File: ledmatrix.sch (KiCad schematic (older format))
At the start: 62 parts, among them U58 sled1735

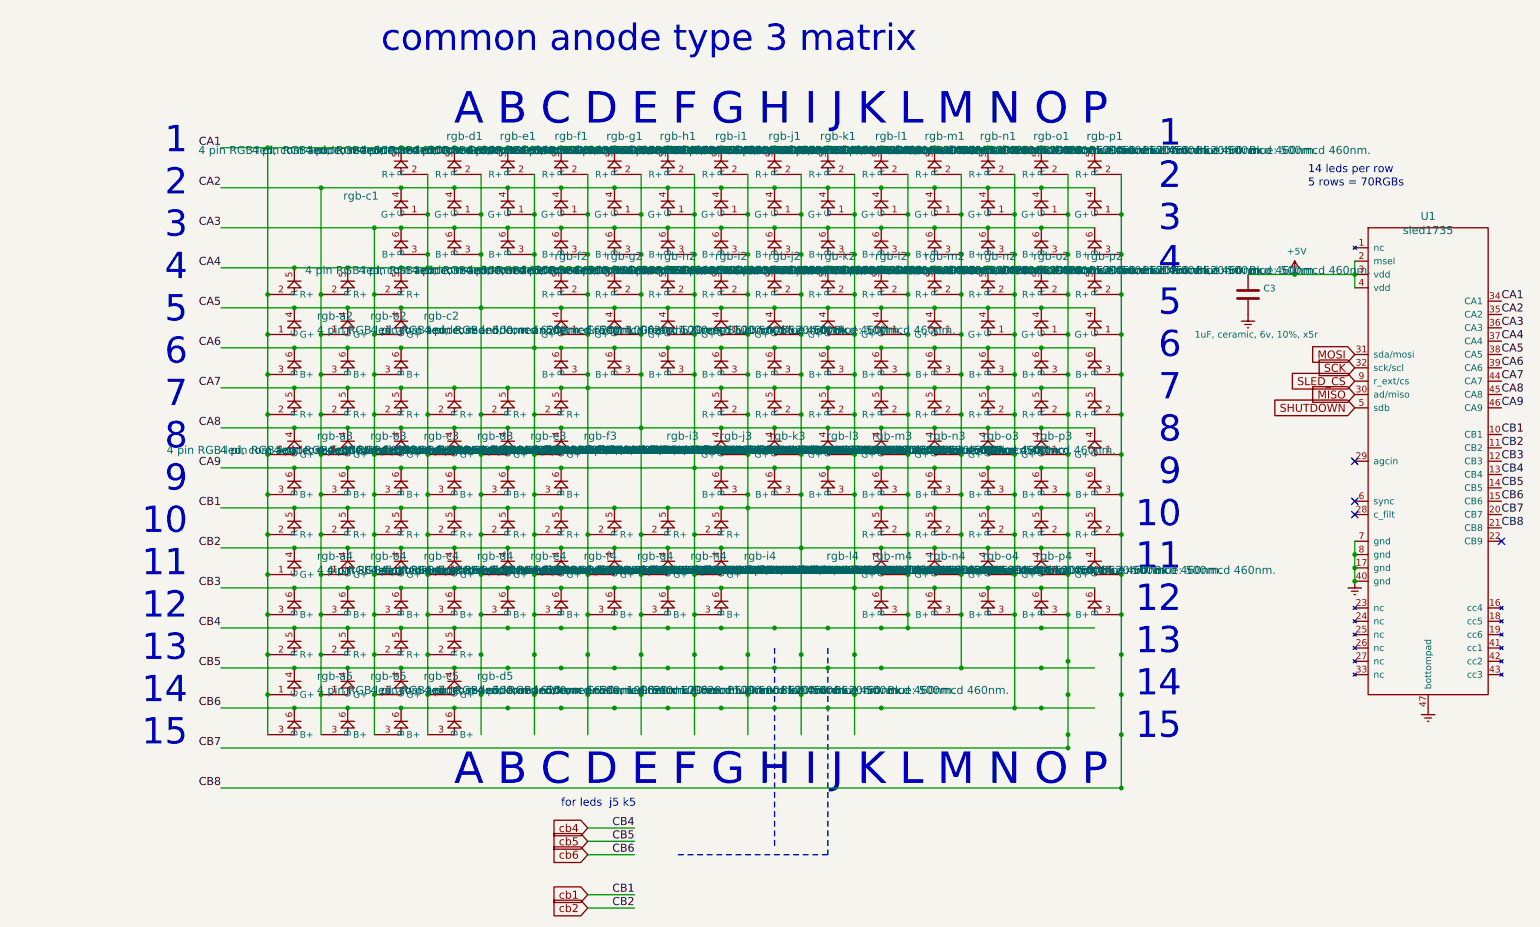
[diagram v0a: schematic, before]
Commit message: ansi/iso work in progress
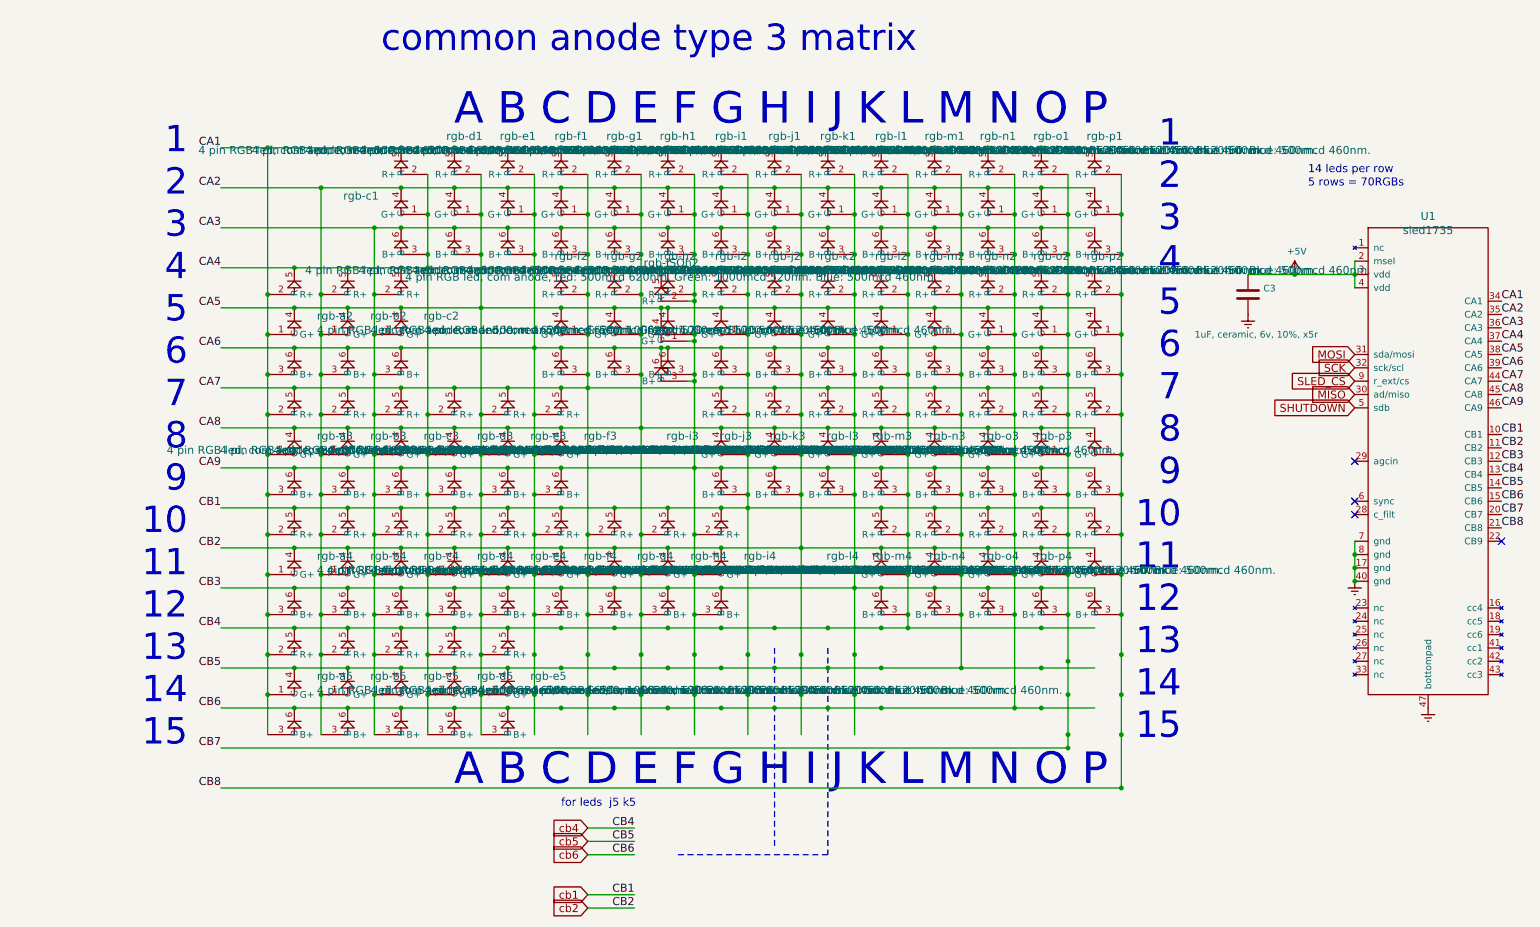
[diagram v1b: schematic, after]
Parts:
- added rgb-ISOh2, rgb-e5: 4 pin RGB led, com anode, red: 500mcd 620nm. Gree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, fp:3528-4p, symbol rgbled
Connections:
- wire segments 42 -> 48
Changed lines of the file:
@@
 Connection ~ 2150 3600
 Connection ~ 1750 3600
+$Comp
+L rgbled rgb-e5
+U 1 1 5AE323BB
+P 3150 5100
+F 0 "rgb-e5" H 2981 5239 60  0000 R CNN
+F 1 "4 pin RGB led, com anode, red: 500mcd 620nm. Green: 1000mcd 520nm. Blue: 500mcd 460nm." H 2981 5133 60  0000 R CNN
+F 2 "fp:3528-4p" H 3150 5100 60  0001 C CNN
+F 3 "" H 3150 5100 60  0001 C CNN
+F 4 "any/open" H 400 0   60  0001 C CNN "supplier"
+F 5 "Value" H 3150 5100 60  0001 C CNN "supplier PN"
+F 6 "Value" H 3150 5100 60  0001 C CNN "MOQ"
+F 7 "Value" H 3150 5100 60  0001 C CNN "leadtime"
+	1    3150 5100
+	-1   0    0    -1
+$EndComp
+$Comp
+L rgbled rgb-ISOh2
+U 1 1 5AE32BA1
+P 4300 2450
+F 0 "rgb-ISOh2" H 4375 3037 60  0000 C CNN
+F 1 "4 pin RGB led, com anode, red: 500mcd 620nm. Green: 1000mcd 520nm. Blue: 500mcd 460nm." H 4375 2931 60  0000 C CNN
+F 2 "fp:3528-4p" H 4300 2450 60  0001 C CNN
+F 3 "" H 4300 2450 60  0001 C CNN
+F 4 "any/open" H -50 50  60  0001 C CNN "supplier"
+F 5 "Value" H 4300 2450 60  0001 C CNN "supplier PN"
+F 6 "Value" H 4300 2450 60  0001 C CNN "MOQ"
+F 7 "Value" H 4300 2450 60  0001 C CNN "leadtime"
+	1    4300 2450
+	1    0    0    -1
+$EndComp
+Wire Wire Line
+	4300 2250 4300 2200
+Connection ~ 4300 2200
+Wire Wire Line
+	4300 1950 4300 1900
+Connection ~ 4300 1900
+Wire Wire Line
+	4300 2550 4300 2500
+Connection ~ 4300 2500
+Wire Wire Line
+	4500 2450 4550 2450
+Connection ~ 4550 2450
+Wire Wire Line
+	4500 2150 4550 2150
+Connection ~ 4550 2150
+Wire Wire Line
+	4500 2750 4550 2750
+Connection ~ 4550 2750
 $EndSCHEMATC
